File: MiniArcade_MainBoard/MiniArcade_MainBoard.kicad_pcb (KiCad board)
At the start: 2 copper layers, 55.5 x 42 mm, 30 parts, among them J1 62701021721, J2 Conn_01x05_Pin, J3 Conn_01x06_Pin, J4 F3311A7H121026E200, SW1 EVPAA, U1 ATSAMD21J18A-A, U2 LM321

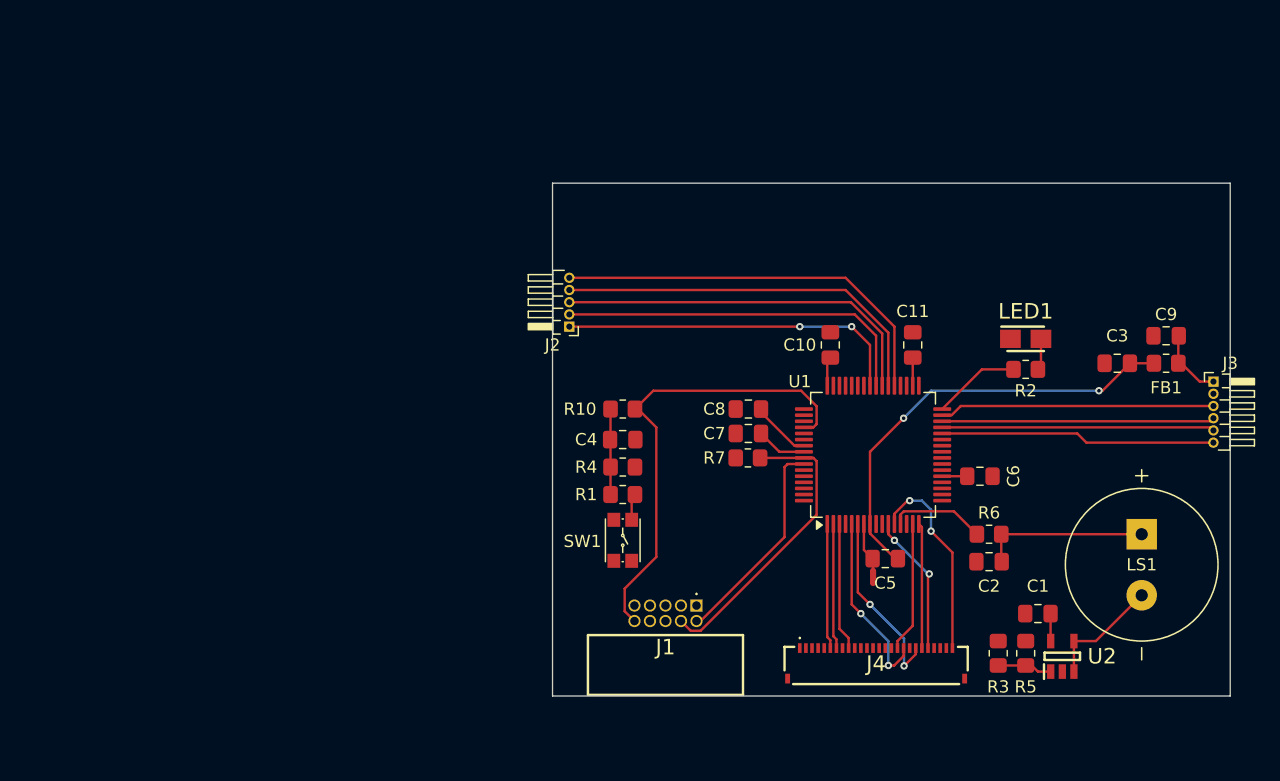
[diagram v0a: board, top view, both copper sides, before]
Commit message: 11 11 2025
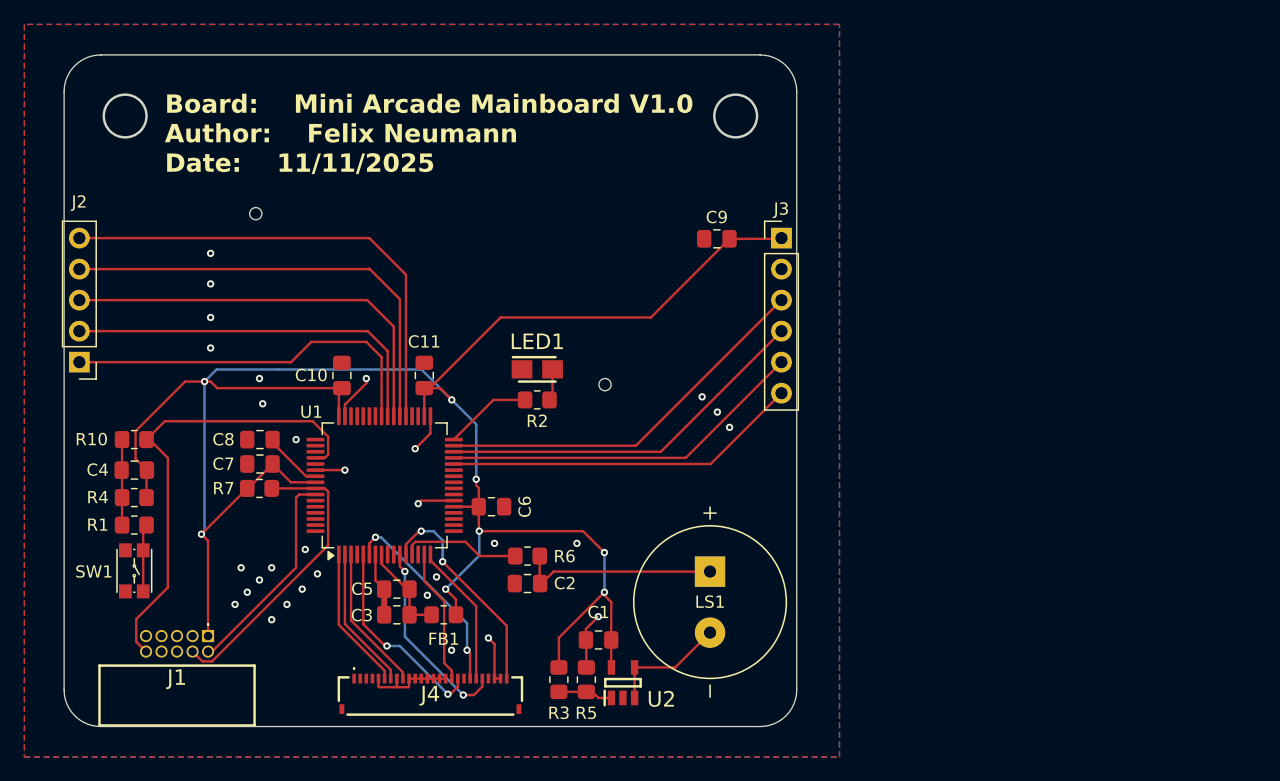
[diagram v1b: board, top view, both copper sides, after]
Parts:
- added U3: ~, MainBoard:ERTFT144, B.Cu at (155.3, 95.2)
- J2: footprint Connector_PinHeader_1.00mm:PinHeader_1x05_P1.00mm_Horizontal -> Connector_PinHeader_2.54mm:PinHeader_1x05_P2.54mm_Vertical
- J3: footprint Connector_PinHeader_1.00mm:PinHeader_1x06_P1.00mm_Horizontal -> Connector_PinHeader_2.54mm:PinHeader_1x06_P2.54mm_Vertical
- moved FB1 62.6 mm to (141.1, 135.8)
- moved C3 62.5 mm to (137.2, 135.8)
- moved J2 40.2 mm to (111.2, 115.2)
- moved NT1 40.1 mm to (136.2, 134.8)
- moved C10 40.1 mm to (132.8, 116.2)
- moved C11 40.1 mm to (139.5, 116.2)
- moved C4 40.1 mm to (115.8, 124.0)
- moved C5 40.1 mm to (137.2, 133.8)
- moved C6 40.1 mm to (145.0, 127.0)
- moved C7 40.1 mm to (126.0, 123.5)
- moved C8 40.1 mm to (126.0, 121.5)
- moved LED1 40.1 mm to (148.8, 115.8)
- moved R1 40.1 mm to (115.8, 128.5)
- moved R10 40.1 mm to (115.8, 121.5)
- moved R2 40.1 mm to (148.8, 118.2)
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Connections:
- C4 pad 1: 3.3V -> 3V3
- R4 pad 1: 3.3V -> 3V3
- R7 pad 2: +3.3V -> 3V3
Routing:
- net 3V3: track 19.0 -> 172.4 mm, vias 0 -> 8
- net GND: track 0.00 -> 29.2 mm, vias 0 -> 31
- net VDDANA: track 36.1 -> 7.82 mm, vias 2 -> 0
- net DP_UP: track 22.5 -> 31.8 mm
- net DP_RIGHT: track 22.3 -> 30.9 mm
- net DP_DOWN: track 22.3 -> 30.1 mm
- net DP_LEFT: track 22.5 -> 29.2 mm
- net JS_RIGHT: track 33.2 -> 39.6 mm
- net JS_SWITCH: track 31.9 -> 36.9 mm
- net CS: track 11.7 -> 16.2 mm
- net Net-(R1-Pad1): track 2.18 -> 5.54 mm
- net JS_DOWN: track 31.0 -> 34.1 mm
- net Net-(C2-Pad2): track 13.8 -> 16.6 mm
- net JS_UP: track 28.8 -> 30.9 mm, vias 2 -> 0
- net BUZZER: track 7.91 -> 9.81 mm
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- added copper zone on B.Cu, net GND
- added copper zone on F.Cu, net GND
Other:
- board size 55.5 x 42 mm -> 60 x 55 mm
- board text added: "Board: Mini Arcade Mainboard V1.0 Author: Felix Neumann Date: 11/11/2025"
